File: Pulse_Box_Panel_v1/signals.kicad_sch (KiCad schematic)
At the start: 25 parts, among them J1 Conn_01x11, J2 Conn_01x11, J3 Conn_01x11, J4 Conn_01x11, J5 Conn_01x03, J6 Conn_01x03, J8 Conn_01x03, J9 Conn_02x05_Odd_Even, U1 STM32G0B1CBTx, U4 74HCT4051, U5 74HCT4051, Y1 8MHz Crystal

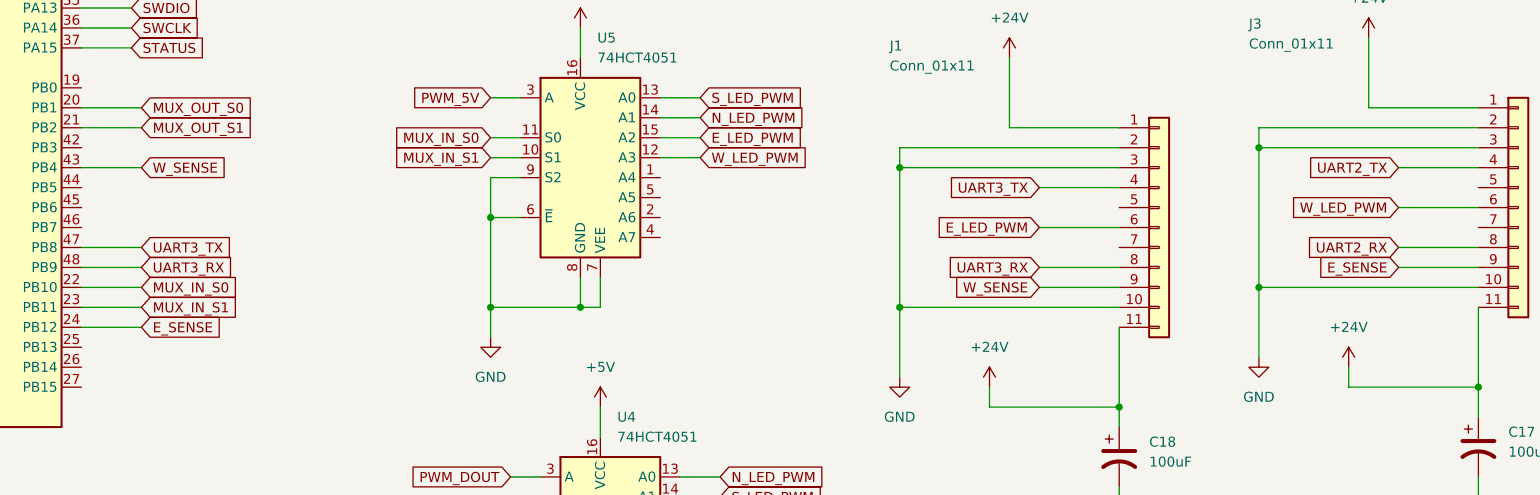
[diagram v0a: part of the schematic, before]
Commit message: basic readme with board summaries
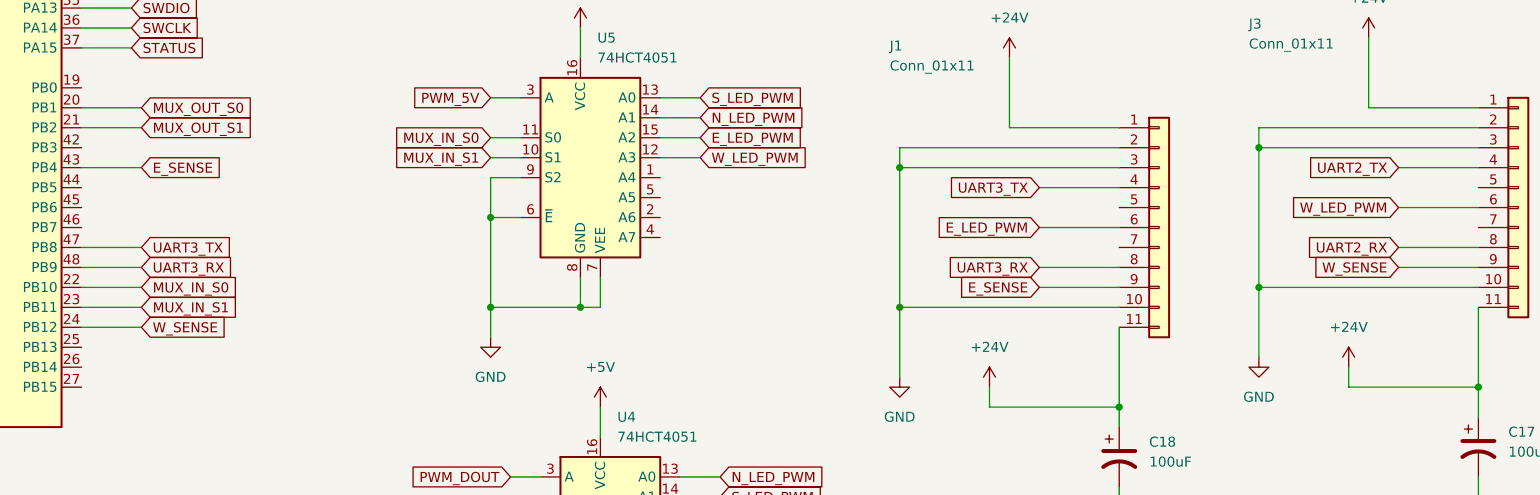
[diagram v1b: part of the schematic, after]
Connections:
- net E_SENSE: now also J1.9 (Pin_9), U1.43 (PB4); no longer J3.9 (Pin_9), U1.24 (PB12)
- net W_SENSE: now also J3.9 (Pin_9), U1.24 (PB12); no longer J1.9 (Pin_9), U1.43 (PB4)
